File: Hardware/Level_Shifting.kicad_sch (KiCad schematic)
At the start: 28 parts, among them J10 SMA_Edge, J11 SMA_Edge, SW4 SPDT_Slide_SMD_7.2x3.5mm, U10 74LVC2T45DC, U12 74LVC2T45DC, U14 74LVC2T45DC, U15 74LVC2T45DC, U8 74LVC2T45DC, U9 74LVC2T45DC

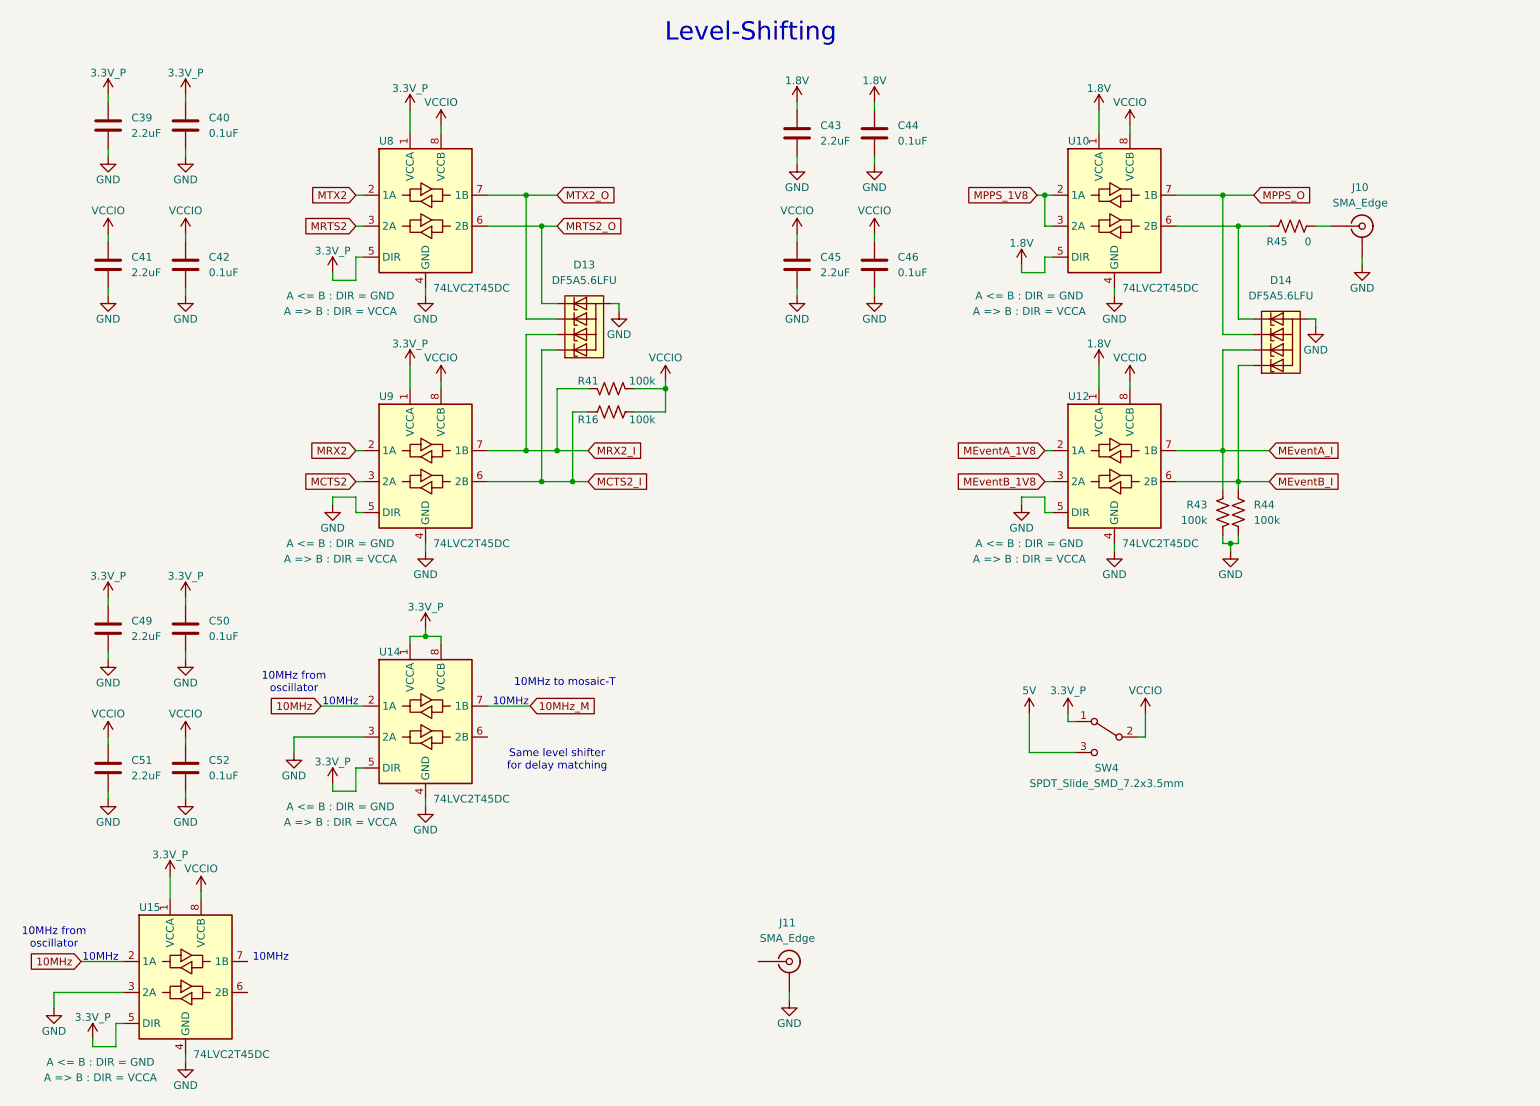
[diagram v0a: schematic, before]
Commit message: Schematic complete
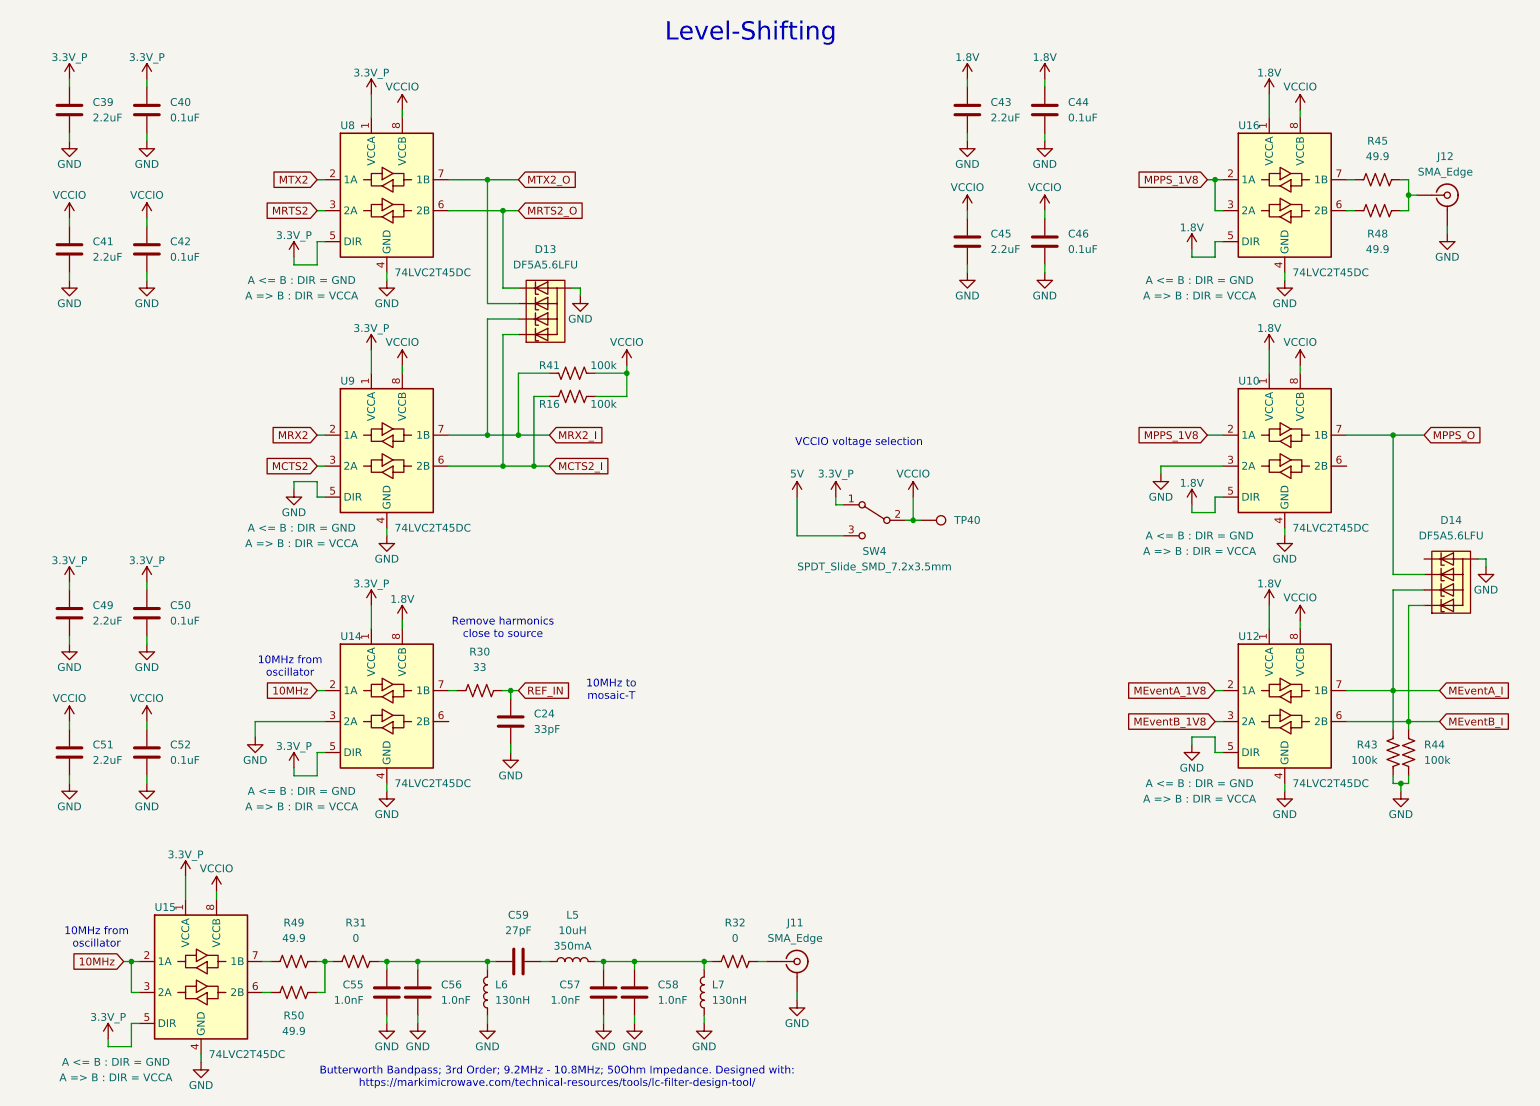
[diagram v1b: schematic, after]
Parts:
- removed J10: SMA_Edge, SparkFun-Connector:SMA_Edge, symbol SparkFun-RF:SMA_EdgeMount
- removed R45: 0, SparkFun-Resistor:R_0603_1608Metric, symbol SparkFun-Resistor:0_0603
- added C24: 33pF, SparkFun-Capacitor:C_0603_1608Metric, symbol SparkFun-Capacitor:33pF_0603_50V_5%
- added C55, C56, C57, C58: 1.0nF, SparkFun-Capacitor:C_0603_1608Metric, symbol SparkFun-Capacitor:1.0nF_0603_50V_10%
- added C59: 27pF, SparkFun-Capacitor:C_0603_1608Metric, symbol SparkFun-Capacitor:27pF_0603_50V_5%
- added J12: SMA_Edge, SparkFun-Connector:SMA_Edge, symbol SparkFun-RF:SMA_EdgeMount
- added L5: 10uH, SparkFun-Capacitor:C_0805_2012Metric, symbol SparkFun-Coil:10uH_0805_0.35A
- added L6, L7: 130nH, SparkFun-Capacitor:C_0603_1608Metric, symbol SparkFun-Coil:130nH_0603_170mA
- added R30: 33, SparkFun-Resistor:R_0603_1608Metric, symbol SparkFun-Resistor:33_0603
- added R31, R32: 0, SparkFun-Resistor:R_0603_1608Metric, symbol SparkFun-Resistor:0_0603
- added R45, R48, R49, R50: 49.9, SparkFun-Resistor:R_0603_1608Metric, symbol SparkFun-Resistor:49.9_0603
- added TP40: PTH, SparkFun-Connector:1x01, symbol SparkFun-Connector:TestPoint_PTH
- added U16: 74LVC2T45DC, SparkFun-Semiconductor-Standard:VSSOP8_SOT765-1, symbol SparkFun-IC-Logic:74LVC2T45DC
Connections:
- net 1.8V: now also U14.8 (VCCB), U16.1 (VCCA), U16.5 (DIR)
- net 10MHz: now also U15.3 (2A)
- net 3.3V_P: no longer U14.8 (VCCB)
- net GND: now also U10.3 (2A), C24.2, C55.2, C56.2, C57.2, C58.2, J12.2 (Ext), L6.1, L7.1, U16.4 (GND); no longer U15.3 (2A)
- net MPPS_1V8: now also U16.2 (1A), U16.3 (2A); no longer U10.3 (2A)
- net VCCIO: now also TP40.1, U16.8 (VCCB)
- net at D14.5 (K4): no longer U10.6 (2B)
- net at U15.6 (2B): now also R50.2
- net at U15.7 (1B): now also R49.2
- net at J11.1 (In): now also R32.1
- net 10MHz_M: no longer names the net of U14.7 (1B)
- net 10MHz_M: now also R30.2
- new net: R31.2, R49.1, R50.1
- new net: J12.1 (In), R45.1, R48.1
- new net: C55.1, C56.1, C59.1, L6.2, R31.1
- new net: R45.2, U16.7 (1B)
- new net: C57.1, C58.1, L5.2, L7.2, R32.2
- new net: R48.2, U16.6 (2B)
- new net: C59.2, L5.1
- new net REF_IN: C24.1, R30.1
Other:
- note added: "Butterworth Bandpass; 3rd Order; 9.2MHz - 10.8MHz; 50Ohm Impedance. Designed with: https://markimicrowave.com/technical-resources/tools/lc-filter-design-tool/"
- note added: "Remove harmonics close to source"
- note added: "VCCIO voltage selection"
- note removed: "10MHz"
- note removed: "Same level shifter for delay matching"
- moved on the sheet: C39, C40, C41, C42, C43, C44, C45, C46, C49, C50, C51, C52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
